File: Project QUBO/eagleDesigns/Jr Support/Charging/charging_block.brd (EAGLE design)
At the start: 160 x 100 mm, 120 parts

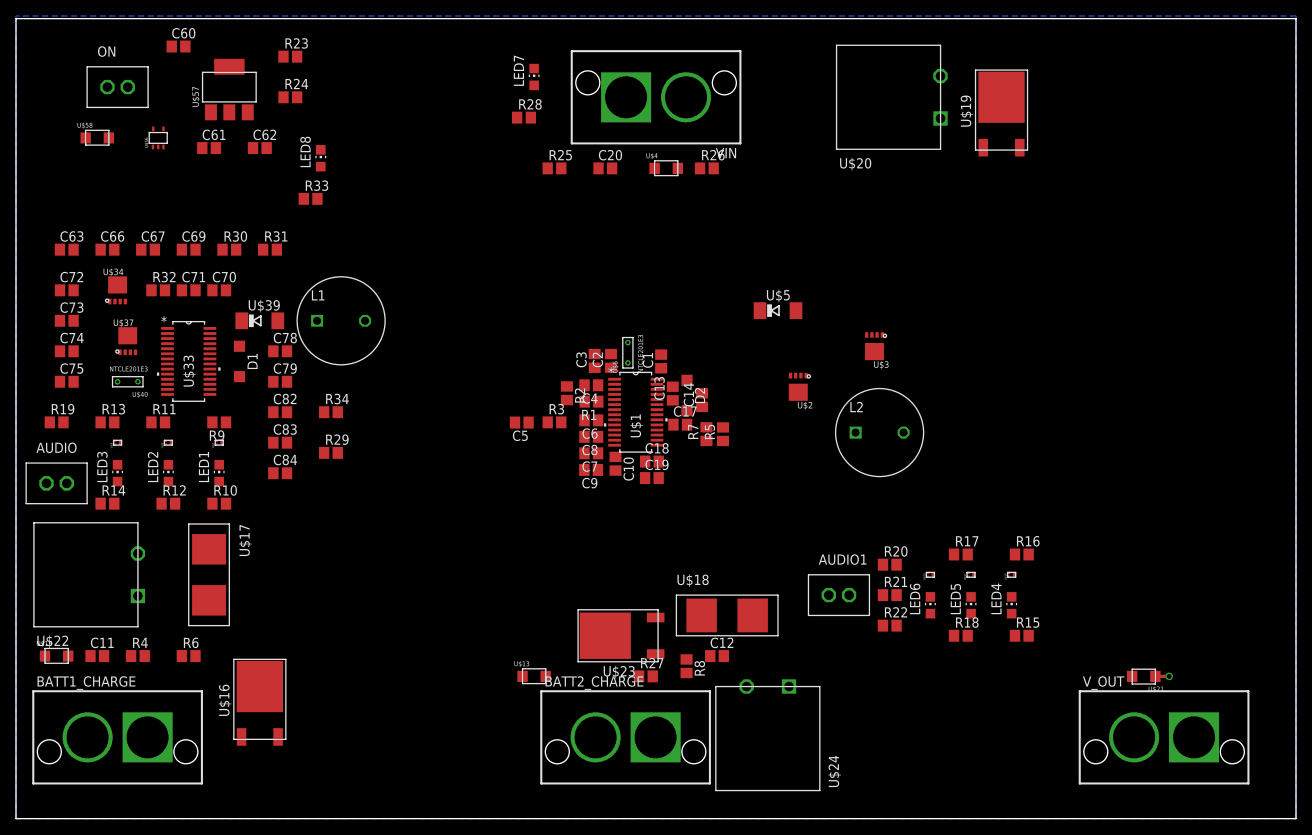
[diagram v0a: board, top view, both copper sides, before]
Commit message: Charging board layout, rev. 1
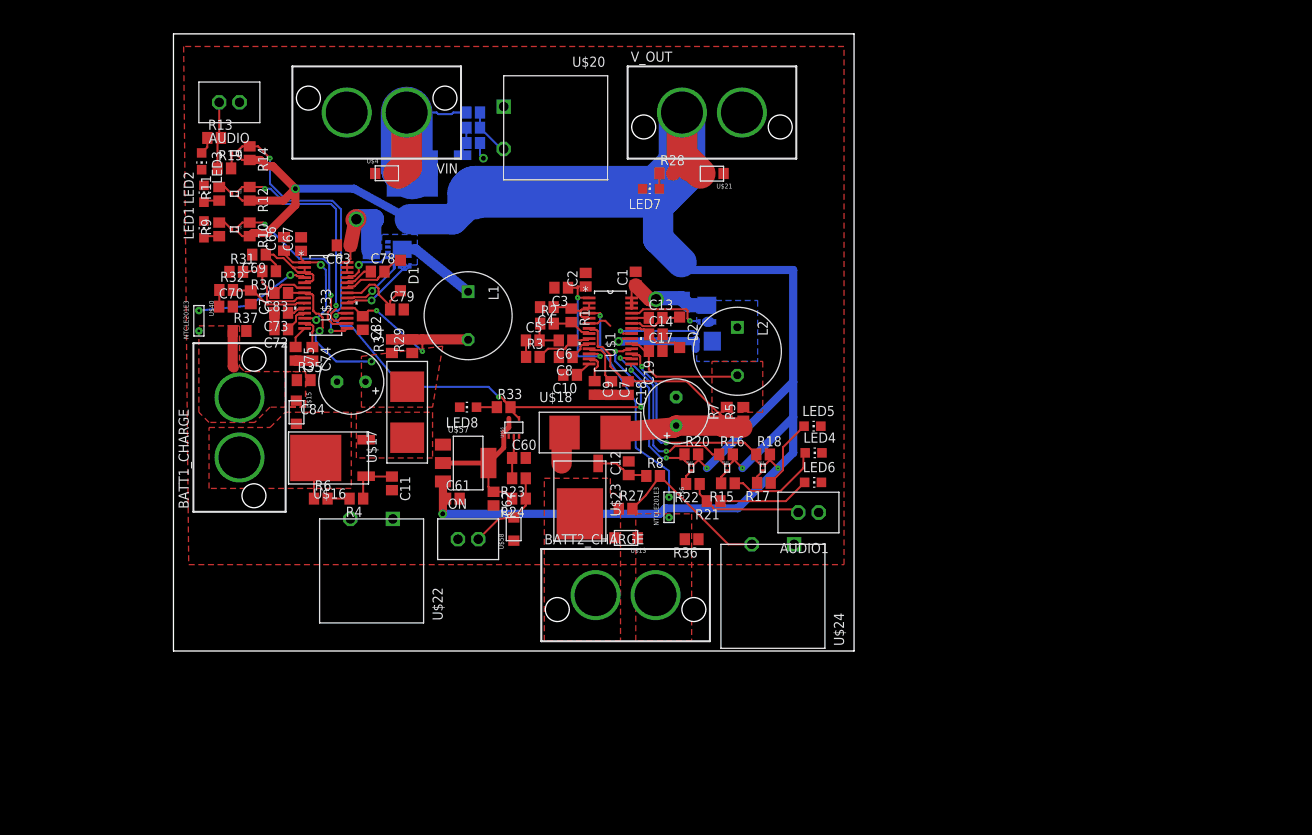
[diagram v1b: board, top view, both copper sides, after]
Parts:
- added R35, R36, R37: 0, resistor:R0805
- C19: value 100u,<50mO -> 120uF; device resistor:C0805 -> resistor:E3,5-8
- C84: value 100u,<50mO -> 120u; device resistor:C0805 -> resistor:E3,5-8
- R28: value 330 -> 1.5k
- moved V_OUT 96.4 mm to (87.0, 88.3)
- moved U$21 82.9 mm to (87.0, 80.6)
- moved U$19 74.3 mm to (49.5, 80.6), flipped to the bottom, turned to 270 degrees
- moved ON 71.5 mm to (56.5, 34.9)
- moved U$58 71.4 mm to (62.2, 36.2), turned to 90 degrees
- moved C60 66.8 mm to (62.9, 45.1)
- moved R23 60.0 mm to (62.9, 42.5), turned to 180 degrees
- moved R24 57.7 mm to (62.9, 40.0), turned to 180 degrees
- moved U$56 57.3 mm to (62.2, 48.9)
- moved U$57 55.7 mm to (56.5, 44.5), turned to 270 degrees
- moved U$20 54.7 mm to (61.0, 86.4), turned to 180 degrees
- moved C61 53.4 mm to (54.6, 40.0)
- moved C62 52.7 mm to (59.7, 40.0), turned to 270 degrees
- moved AUDIO 52.3 mm to (26.7, 89.5), turned to 180 degrees
- moved R14 47.3 mm to (29.2, 83.2), turned to 270 degrees
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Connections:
- net N$11 renamed BATT1_P
- net N$15 renamed DLO_2
- net N$16 renamed DHI_2
- net N$17 renamed L-IN_2
- net N$18 renamed PGND_2
- net N$20 renamed CS_2
- net N$21 renamed THM_2
- net N$42 renamed DCIN_2
- net N$43 renamed BATT2_P
- net N$45 renamed VIN
- net N$46 renamed FET-G_1
- net N$56 renamed FET-D_1
- net N$77 renamed CS_1
- removed net N$48: C60.2, ON.P$2, U$56.P$3, U$58.P$1
- removed net V_BATT1: C83.1, C84.1, R29.1, R34.1, U$17.P$2, U$33.7
- removed net V_BATT2: C18.1, C19.1, R5.1, R7.1, U$1.7, U$18.P$2
- new net BATT1_M: BATT1_CHARGE.P$2, R35.1, R37.1, U$15.P$1, U$40.P$2
- new net BATT2_M: BATT2_CHARGE.P$2, R36.2, U$13.P$1, U$6.P$2
- new net BATT_1: C83.1, C84.+, R29.1, R34.1, U$17.P$2, U$33.7
- new net BATT_2: C18.1, C19.+, R5.1, R7.1, U$1.7, U$18.P$2
- net !SHDN!: now also R33.2
- net GND: now also C19.-, C60.2, C84.-, ON.P$2, R35.2, R36.1, R37.2, U$56.P$3, U$58.P$1; no longer BATT1_CHARGE.P$2, BATT2_CHARGE.P$2, C19.2, C84.2, U$13.P$1, U$15.P$1, U$40.P$2, U$6.P$2
- net V_SHORE: now also R28.2
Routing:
- net V_SHORE: track 0.00 -> 241.1 mm, vias 0 -> 5
- net !SHDN!: track 0.00 -> 58.3 mm, vias 0 -> 4
- net BATT_2: track 0.00 -> 41.8 mm
- net N$31: track 0.00 -> 36.5 mm, vias 0 -> 2
- net N$27: track 0.00 -> 29.9 mm, vias 0 -> 2
- net THM_2: track 0.00 -> 27.8 mm, vias 0 -> 1
- net N$32: track 0.00 -> 27.2 mm, vias 0 -> 2
- net N$38: track 0.00 -> 25.5 mm, vias 0 -> 2
- net N$24: track 0.00 -> 23.7 mm, vias 0 -> 2
- net VIN: track 0.00 -> 23.7 mm
- net CS_1: track 0.00 -> 23.1 mm, vias 0 -> 2
- net N$55: track 0.00 -> 20.4 mm
- net GND: track 2.36 -> 22.4 mm
- net BATT_1: track 0.00 -> 19.0 mm, vias 0 -> 2
- net N$54: track 0.00 -> 18.9 mm
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- added copper zone on layer 1, net BATT1_M
- added copper zone on layer 1, net BATT1_P
- added copper zone on layer 1, net BATT2_M
- added copper zone on layer 1, net BATT2_P
- added copper zone on layer 1, net BATT_1
- added copper zone on layer 1, net CS_2
- added copper zone on layer 1, net FET-D_1
- added copper zone on layer 1, net GND
- added copper zone on layer 16, net L-IN_2
- added copper zone on layer 16, net N$81
- removed copper zone on layer 16, net GND
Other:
- board size 160 x 100 mm -> 85.1 x 77.1 mm
